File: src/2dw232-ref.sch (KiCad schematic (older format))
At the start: 22 parts, among them P501 CONN_01X07, Q501 2N3904, Q502 2N3904, U501 LM741, U502 LM741

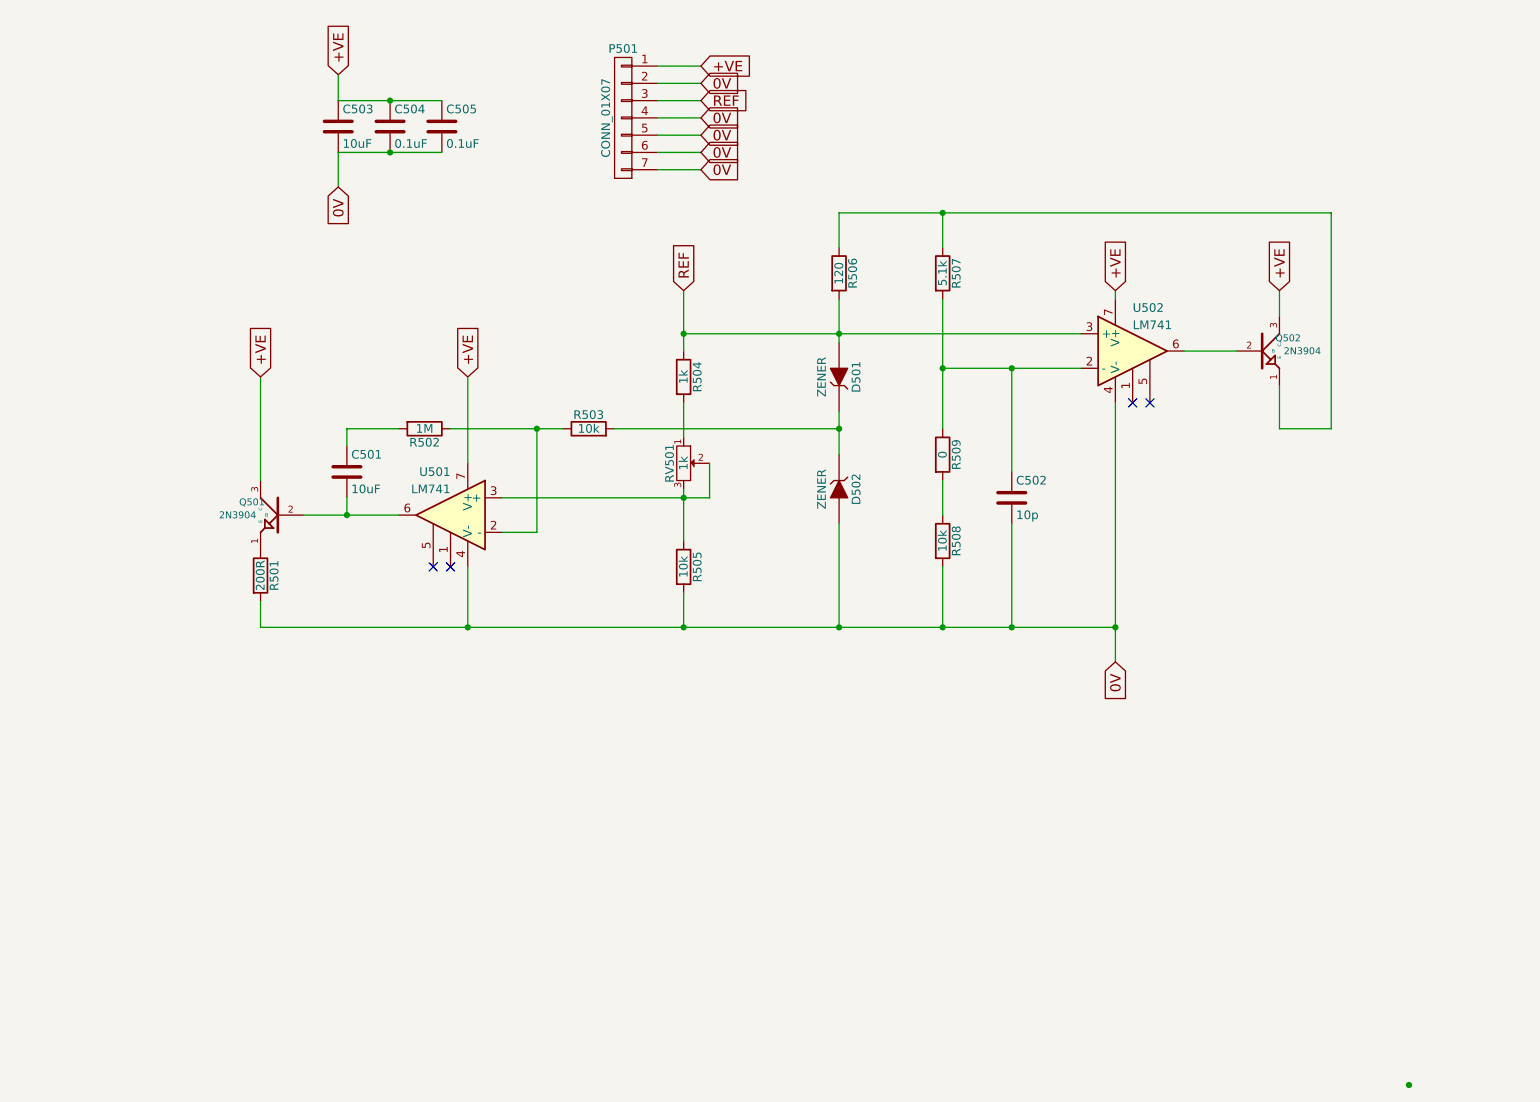
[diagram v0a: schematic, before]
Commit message: 4 layer
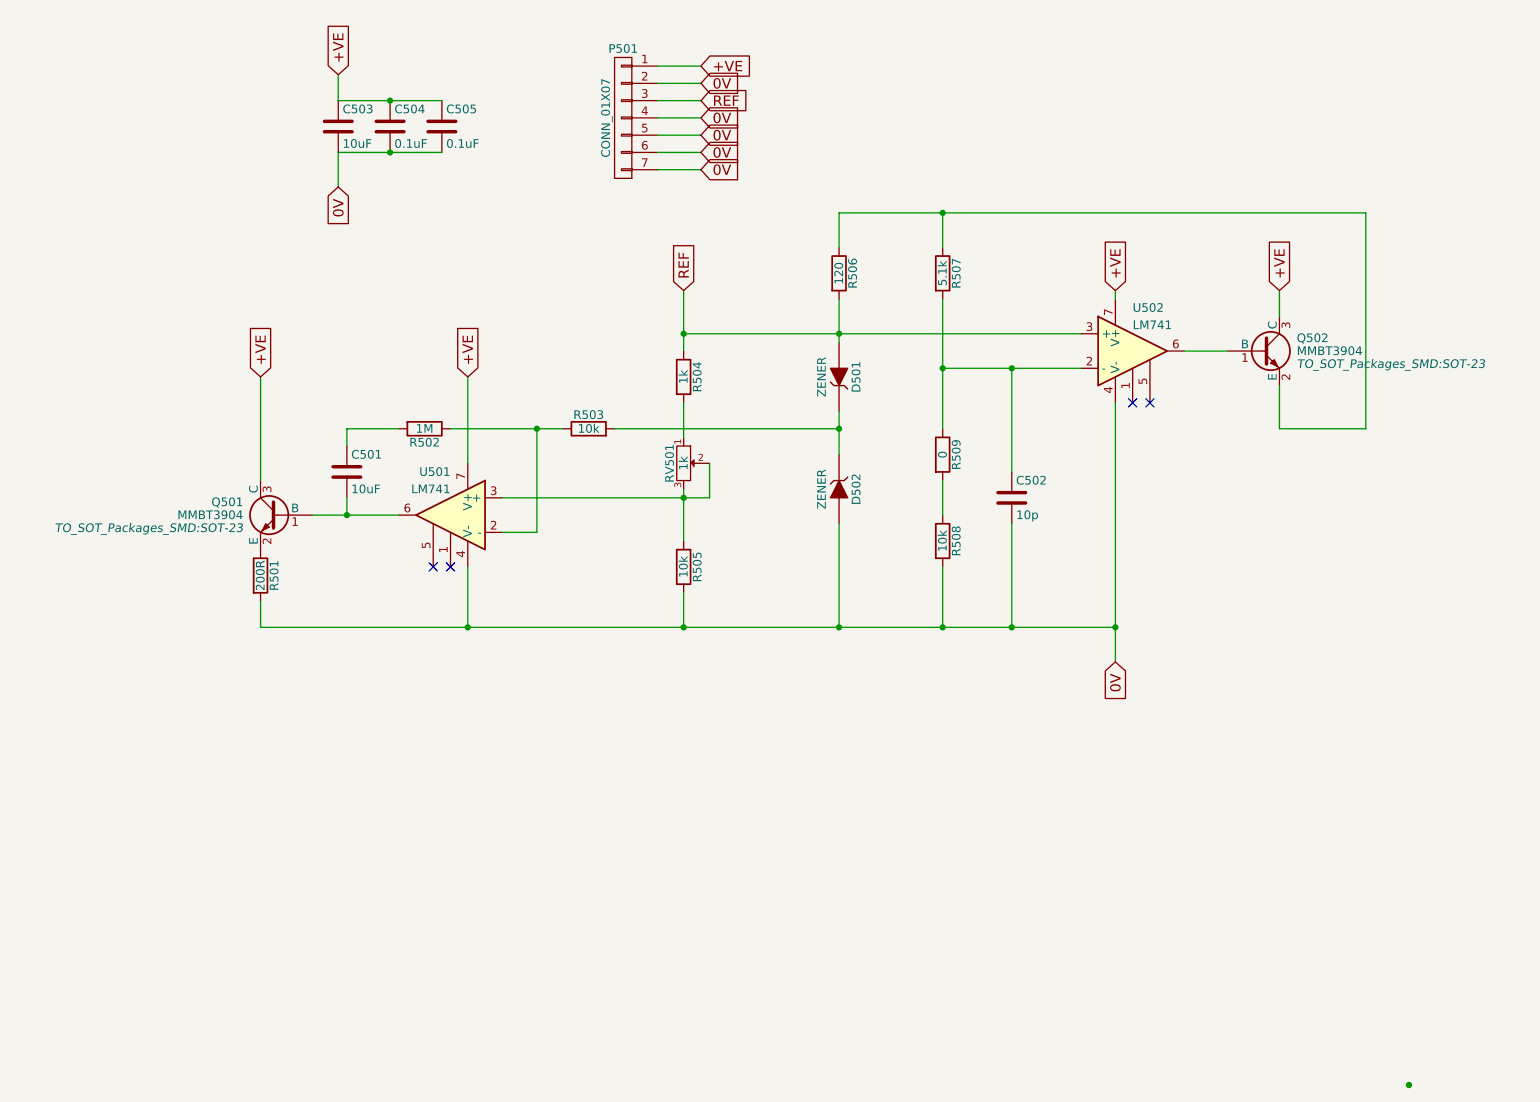
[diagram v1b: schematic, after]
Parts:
- removed Q501, Q502: 2N3904, TO_SOT_Packages_SMD:SOT-23, symbol 2N3904
- added Q501, Q502: MMBT3904, TO_SOT_Packages_SMD:SOT-23, symbol MMBT3904
- R504, R505, R506, R507, R508, R509: footprint Resistors_ThroughHole:Resistor_Horizontal_RM7mm -> Resistors_ThroughHole:Resistor_TO-220_Vertical
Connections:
- net +VE: now also Q501.3 (C), Q502.3 (C)
- net at U502.6: now also Q502.1 (B)
- net at R506.1, R507.1: now also Q502.2 (E)
- net at C501.2, U501.6: now also Q501.1 (B)
- net at R501.1: now also Q501.2 (E)
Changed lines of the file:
@@
 F 0 "R508" V 5430 3650 50  0000 C CNN
 F 1 "10k" V 5350 3650 50  0000 C CNN
-F 2 "Resistors_ThroughHole:Resistor_Horizontal_RM7mm" V 5280 3650 50  0001 C CNN
+F 2 "Resistors_ThroughHole:Resistor_TO-220_Vertical" V 5280 3650 50  0001 C CNN
 F 3 "" H 5350 3650 50  0000 C CNN
 	1    5350 3650
@@
 F 0 "R507" V 5430 2100 50  0000 C CNN
 F 1 "5.1k" V 5350 2100 50  0000 C CNN
-F 2 "Resistors_ThroughHole:Resistor_Horizontal_RM7mm" V 5280 2100 50  0001 C CNN
+F 2 "Resistors_ThroughHole:Resistor_TO-220_Vertical" V 5280 2100 50  0001 C CNN
 F 3 "" H 5350 2100 50  0000 C CNN
 	1    5350 2100
@@
 $EndComp
 Wire Wire Line
-	7050 2550 6750 2550
-Wire Wire Line
-	4750 1750 7600 1750
+	4750 1750 7800 1750
 Wire Wire Line
 	5350 1750 5350 1950
@@
 F 0 "R506" V 4830 2100 50  0000 C CNN
 F 1 "120" V 4750 2100 50  0000 C CNN
-F 2 "Resistors_ThroughHole:Resistor_Horizontal_RM7mm" V 4680 2100 50  0001 C CNN
+F 2 "Resistors_ThroughHole:Resistor_TO-220_Vertical" V 4680 2100 50  0001 C CNN
 F 3 "" H 4750 2100 50  0000 C CNN
 	1    4750 2100
@@
 Connection ~ 5350 1750
 Connection ~ 4750 2450
-$Comp
-L 2N3904 Q502
-U 1 1 588188E4
-P 7200 2550
-F 0 "Q502" H 7350 2625 40  0000 C CNN
-F 1 "2N3904" H 7325 2550 40  0000 L CNN
-F 2 "TO_SOT_Packages_SMD:SOT-23" H 7200 2550 60  0001 C CNN
-F 3 "" H 7200 2550 60  0001 C CNN
-	1    7200 2550
-	1    0    0    -1
-$EndComp
 Text GLabel 7300 2200 1    60   Input ~ 0
 +VE
@@
 F 0 "R504" V 3930 2700 50  0000 C CNN
 F 1 "1k" V 3850 2700 50  0000 C CNN
-F 2 "Resistors_ThroughHole:Resistor_Horizontal_RM7mm" V 3780 2700 50  0001 C CNN
+F 2 "Resistors_ThroughHole:Resistor_TO-220_Vertical" V 3780 2700 50  0001 C CNN
 F 3 "" H 3850 2700 50  0000 C CNN
 	1    3850 2700
@@
 F 0 "R505" V 3930 3800 50  0000 C CNN
 F 1 "10k" V 3850 3800 50  0000 C CNN
-F 2 "Resistors_ThroughHole:Resistor_Horizontal_RM7mm" V 3780 3800 50  0001 C CNN
+F 2 "Resistors_ThroughHole:Resistor_TO-220_Vertical" V 3780 3800 50  0001 C CNN
 F 3 "" H 3850 3800 50  0000 C CNN
 	1    3850 3800
@@
 	1900 3400 1900 3500
 Wire Wire Line
-	1650 3500 2200 3500
+	1700 3500 2200 3500
 Text GLabel 2600 2700 1    60   Input ~ 0
 +VE
@@
 	2600 2700 2600 3200
 Connection ~ 3850 4150
-$Comp
-L 2N3904 Q501
-U 1 1 5881F2EF
-P 1500 3500
-F 0 "Q501" H 1650 3575 40  0000 C CNN
-F 1 "2N3904" H 1625 3500 40  0000 L CNN
-F 2 "TO_SOT_Packages_SMD:SOT-23" H 1500 3500 60  0001 C CNN
-F 3 "" H 1500 3500 60  0001 C CNN
-	1    1500 3500
-	-1   0    0    -1
-$EndComp
 Connection ~ 1900 3500
 Text GLabel 1400 2700 1    60   Input ~ 0
@@
 $EndComp
 Wire Wire Line
-	7600 1750 7600 3000
-Wire Wire Line
-	7600 3000 7300 3000
+	7800 1750 7800 3000
+Wire Wire Line
+	7800 3000 7300 3000
 Wire Wire Line
 	7300 3000 7300 2750
@@
 F 0 "R509" V 5430 3150 50  0000 C CNN
 F 1 "0" V 5350 3150 50  0000 C CNN
-F 2 "Resistors_ThroughHole:Resistor_Horizontal_RM7mm" V 5280 3150 50  0001 C CNN
+F 2 "Resistors_ThroughHole:Resistor_TO-220_Vertical" V 5280 3150 50  0001 C CNN
 F 3 "" H 5350 3150 50  0000 C CNN
 	1    5350 3150
@@
 Wire Wire Line
 	3700 1500 3950 1500
+$Comp
+L MMBT3904 Q502
+U 1 1 58835E41
+P 7200 2550
+F 0 "Q502" H 7400 2625 50  0000 L CNN
+F 1 "MMBT3904" H 7400 2550 50  0000 L CNN
+F 2 "TO_SOT_Packages_SMD:SOT-23" H 7400 2475 50  0000 L CIN
+F 3 "" H 7200 2550 50  0000 L CNN
+	1    7200 2550
+	1    0    0    -1
+$EndComp
+Wire Wire Line
+	7000 2550 6750 2550
+$Comp
+L MMBT3904 Q501
+U 1 1 58836CA2
+P 1500 3500
+F 0 "Q501" H 1700 3575 50  0000 L CNN
+F 1 "MMBT3904" H 1700 3500 50  0000 L CNN
+F 2 "TO_SOT_Packages_SMD:SOT-23" H 1700 3425 50  0000 L CIN
+F 3 "" H 1500 3500 50  0000 L CNN
+	1    1500 3500
+	-1   0    0    -1
+$EndComp
 $EndSCHEMATC
